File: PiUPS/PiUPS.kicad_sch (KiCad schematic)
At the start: 111 parts, among them J1 USB_C_Receptacle_USB2.0, J2 USB_B_Micro, J3 Screw_Terminal_01x02, J4 Raspberry_Pi_2_3, J5 USB_A, Q1 IRF7404, Q2 IRF7404, Q3 IRLML2803TRPBF, Q4 IRF7404, Q5 IRF7404, Q6 IRLML2803TRPBF, Q7 IRLML2803TRPBF, Q8 IRF7404, Q9 IRLML2803TRPBF, SW2 MODE (JS102011SAQN), U1 LM393, U2 BQ25895RTW, U5 TPS61088RHLR, U6 DS3231M

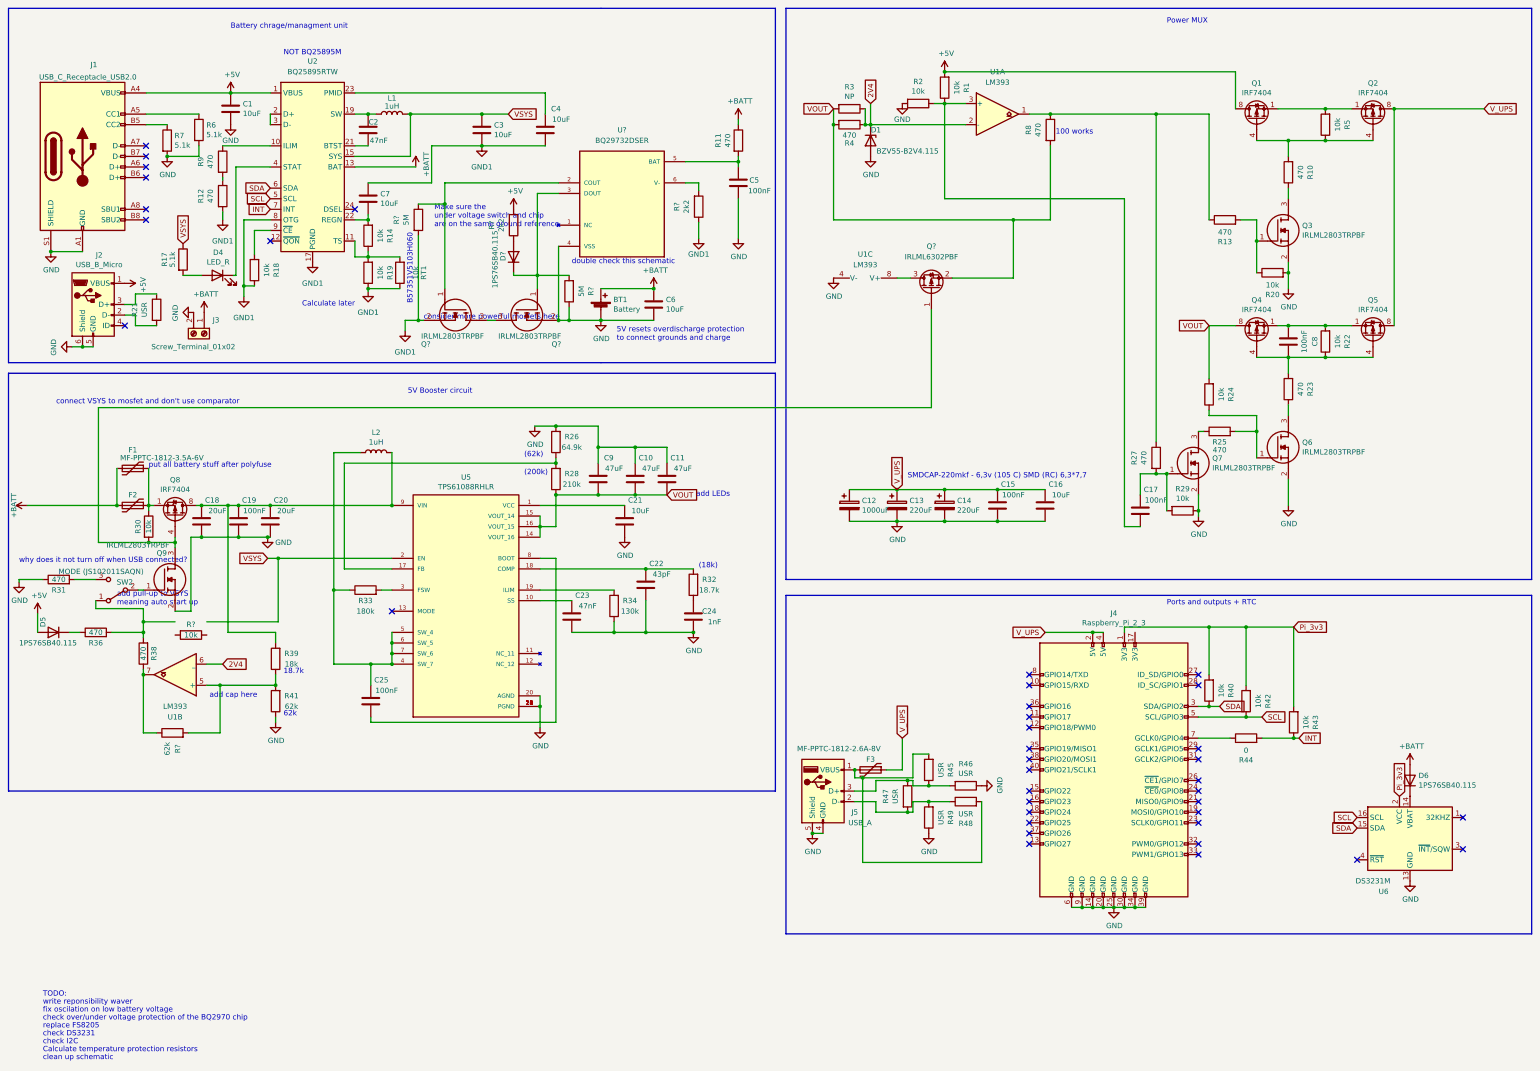
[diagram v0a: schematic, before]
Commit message: minor schematic changes
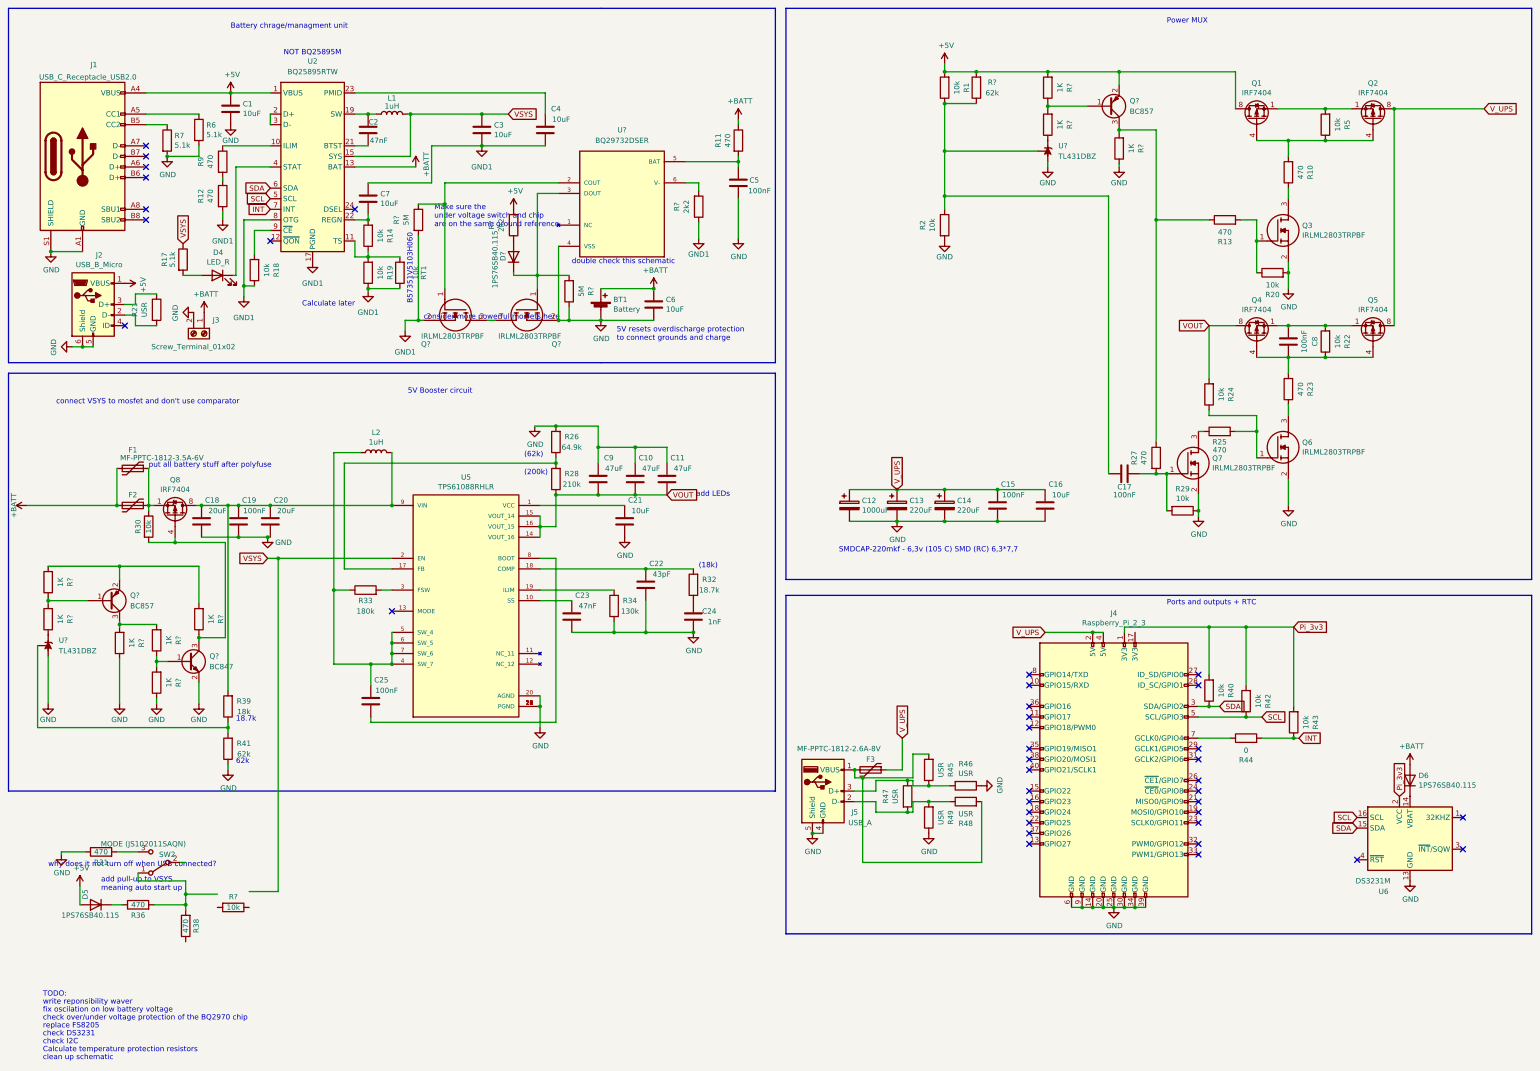
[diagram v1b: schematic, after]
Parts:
- removed D1: BZV55-B2V4.115, Diode_SMD:D_1206_3216Metric_Pad1.42x1.75mm_HandSolder, symbol Device:D_Zener
- removed Q9: IRLML2803TRPBF, IRLML2803TRPBF:SOT95P237X112-3N, symbol IRLML2803TRPBF:IRLML2803TRPBF
- removed Q?: IRLML6302PBF, symbol Device:Q_PMOS_GSD
- removed R3: NP, Resistor_SMD:R_0805_2012Metric_Pad1.20x1.40mm_HandSolder, symbol Device:R
- removed R4, R8: 470, Resistor_SMD:R_0805_2012Metric_Pad1.20x1.40mm_HandSolder, symbol Device:R
- removed R?: 62k, Resistor_SMD:R_0805_2012Metric_Pad1.20x1.40mm_HandSolder, symbol Device:R
- removed U1: LM393, symbol Comparator:LM393
- added Q? (x2): BC857, Package_TO_SOT_SMD:SOT-23, symbol Transistor_BJT:BC857
- added Q?: BC847, Package_TO_SOT_SMD:SOT-23, symbol Transistor_BJT:BC847
- added R? (x9): 1K, Resistor_SMD:R_0805_2012Metric_Pad1.20x1.40mm_HandSolder, symbol Device:R
- added R?: 62k, Resistor_SMD:R_0805_2012Metric_Pad1.20x1.40mm_HandSolder, symbol Device:R
- added U? (x2): TL431DBZ, Package_TO_SOT_SMD:SOT-23, symbol Reference_Voltage:TL431DBZ
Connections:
- net +5V: now also Q?.2 (E), R?.2, R?.2
- net GND: now also Q?.2 (E), R?.1, R?.1, R?.1, U?.3 (A), U?.3 (A)
- net at R13.1, R27.1: now also Q?.3 (C), R?.2
- net at Q7.1, R27.2, R29.2: now also C17.2; no longer C17.1
- net at R1.1, R2.1: now also C17.1, R?.1, U?.2 (REF); no longer C17.2
- net at Q8.4 (G), R30.2: now also Q?.3 (C), R?.1
- net at R39.1, R41.2: now also U?.2 (REF)
- new net: Q?.1 (B), R?.1, R?.2 (x3)
- new net: R?.1, U?.1 (K) (x2)
- new net: Q?.3 (C), R?.2, R?.2
- new net: Q?.2 (E), R?.2, R?.2
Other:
- note removed: "100 works"
- note removed: "add cap here"
- moved on the sheet: C17, D5, R2, R31, R36, R38, R39, R41, R?, SW2
